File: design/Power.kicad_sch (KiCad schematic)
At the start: 77 parts, among them J1 CLIFF_FC68148(DC-10A), J19 TE_641119-2, Q1 BC857BV, Q16 SI4459BDY-T1-GE3, Q2 SI4459BDY-T1-GE3, Q22 BC857BV, Q23 SI4459BDY-T1-GE3, Q4 SI4459BDY-T1-GE3, Q8 BSS138L, Q9 BSS138L, U17 INA219BIDCNT, U18 MYRGC075050R31RA, U32 INA219BIDCNT, U40 AG5300, U41 FOD817DSD, U57 INA219BIDCNT, U62 INA219AIDR, U63 INA219AIDR, U64 INA219AIDR

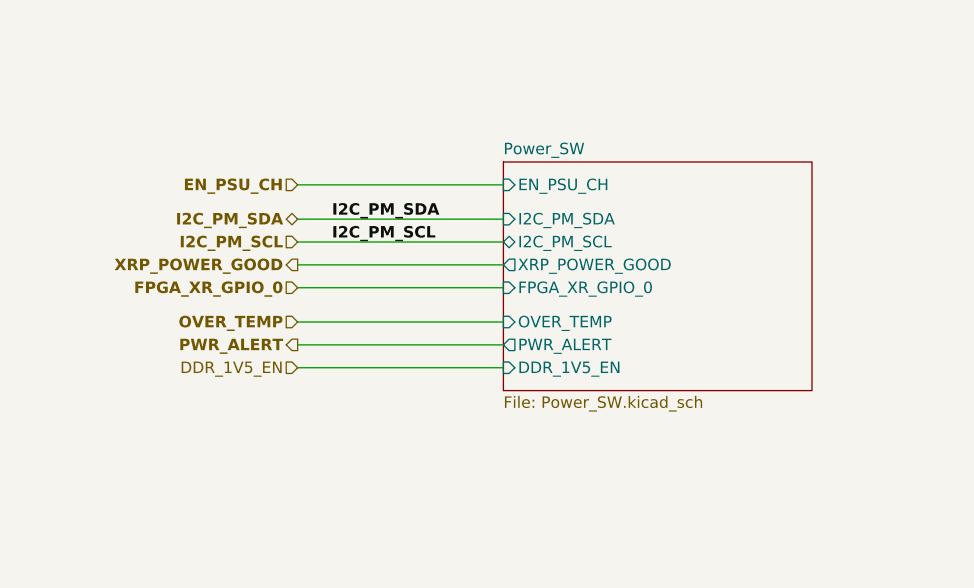
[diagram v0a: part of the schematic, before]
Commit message: no ERC issues
no ERC issues
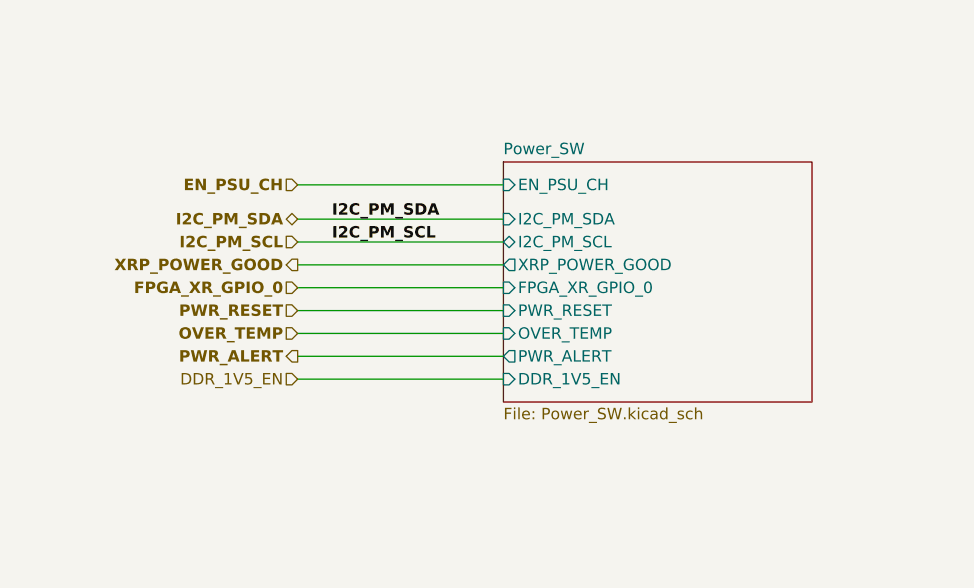
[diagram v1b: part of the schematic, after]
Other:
- sheet Power_SW ports: added PWR_RESET; removed none
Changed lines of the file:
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@@
     (stroke (width 0) (type default) (color 0 0 0 0))
   )
-  (wire (pts (xy 292.1 217.17) (xy 314.96 217.17))
+  (wire (pts (xy 292.1 218.44) (xy 314.96 218.44))
     (stroke (width 0) (type default) (color 0 0 0 0))
   )
@@
     (stroke (width 0) (type default) (color 0 0 0 0))
   )
-  (wire (pts (xy 292.1 212.09) (xy 314.96 212.09))
+  (wire (pts (xy 292.1 210.82) (xy 314.96 210.82))
+    (stroke (width 0) (type default) (color 0 0 0 0))
+  )
+  (wire (pts (xy 292.1 213.36) (xy 314.96 213.36))
     (stroke (width 0) (type default) (color 0 0 0 0))
   )
@@
     (stroke (width 0) (type default) (color 0 0 0 0))
   )
-  (wire (pts (xy 292.1 214.63) (xy 314.96 214.63))
+  (wire (pts (xy 292.1 215.9) (xy 314.96 215.9))
     (stroke (width 0) (type default) (color 0 0 0 0))
   )
@@
     (effects (font (size 1.27 1.27) (thickness 0.254) bold) (justify right))
   )
-  (hierarchical_label "PWR_ALERT" (shape output) (at 292.1 214.63 180)
+  (hierarchical_label "PWR_ALERT" (shape output) (at 292.1 215.9 180)
     (effects (font (size 1.27 1.27) (thickness 0.254) bold) (justify right))
   )
@@
     (effects (font (size 1.27 1.27) (thickness 0.254) bold) (justify right))
   )
-  (hierarchical_label "DDR_1V5_EN" (shape input) (at 292.1 217.17 180)
+  (hierarchical_label "DDR_1V5_EN" (shape input) (at 292.1 218.44 180)
     (effects (font (size 1.27 1.27)) (justify right))
   )
@@
     (effects (font (size 1.27 1.27) (thickness 0.254) bold) (justify right))
   )
-  (hierarchical_label "OVER_TEMP" (shape input) (at 292.1 212.09 180)
+  (hierarchical_label "OVER_TEMP" (shape input) (at 292.1 213.36 180)
+    (effects (font (size 1.27 1.27) (thickness 0.254) bold) (justify right))
+  )
+  (hierarchical_label "PWR_RESET" (shape input) (at 292.1 210.82 180)
     (effects (font (size 1.27 1.27) (thickness 0.254) bold) (justify right))
   )
@@
     (pin "1")
   )
-  (sheet (at 314.96 194.31) (size 34.29 25.4) (fields_autoplaced)
+  (sheet (at 314.96 194.31) (size 34.29 26.67) (fields_autoplaced)
     (stroke (width 0) (type solid) (color 0 0 0 0))
     (fill (color 0 0 0 0.0000))
@@
       (effects (font (size 1.27 1.27)) (justify left bottom))
     )
-    (property "Sheet file" "Power_SW.kicad_sch" (id 1) (at 314.96 220.2946 0)
+    (property "Sheet file" "Power_SW.kicad_sch" (id 1) (at 314.96 221.5646 0)
       (effects (font (size 1.27 1.27)) (justify left top))
     )
@@
       (effects (font (size 1.27 1.27)) (justify left))
     )
-    (pin "OVER_TEMP" input (at 314.96 212.09 180)
+    (pin "OVER_TEMP" input (at 314.96 213.36 180)
       (effects (font (size 1.27 1.27)) (justify left))
     )
-    (pin "DDR_1V5_EN" input (at 314.96 217.17 180)
+    (pin "DDR_1V5_EN" input (at 314.96 218.44 180)
       (effects (font (size 1.27 1.27)) (justify left))
     )
@@
       (effects (font (size 1.27 1.27)) (justify left))
     )
-    (pin "PWR_ALERT" output (at 314.96 214.63 180)
+    (pin "PWR_ALERT" output (at 314.96 215.9 180)
+      (effects (font (size 1.27 1.27)) (justify left))
+    )
+    (pin "PWR_RESET" input (at 314.96 210.82 180)
       (effects (font (size 1.27 1.27)) (justify left))
     )
